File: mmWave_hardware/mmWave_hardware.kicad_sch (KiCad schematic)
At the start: 48 parts, among them J1 Conn_02x08_Top_Bottom, U1 IWRL6432BDBAAMFR, U2 W25Q128JVS, U3 AMS1117-3.3, U4 TPS628502QDRLRQ1, Y1 40.000

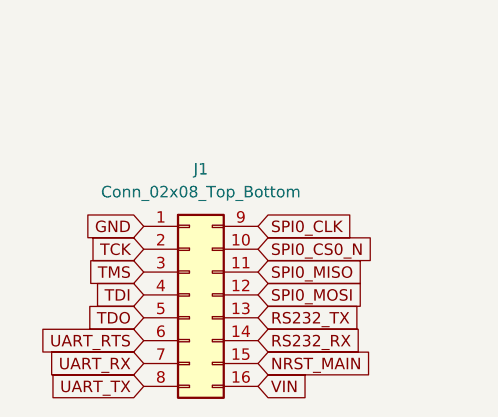
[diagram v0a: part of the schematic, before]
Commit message: PCB Complete
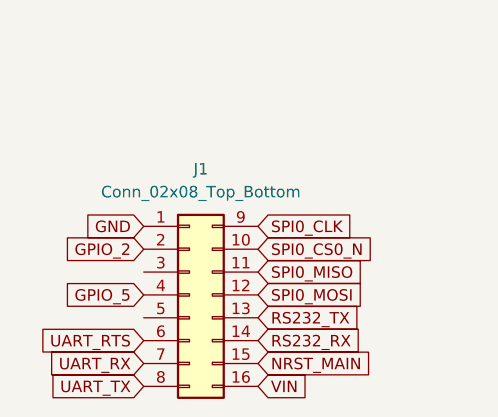
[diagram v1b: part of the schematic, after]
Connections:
- net GPIO_2: now also J1.2 (Pin_2)
- net GPIO_5: now also J1.4 (Pin_4)
- net TCK: no longer J1.2 (Pin_2)
- net TDI: no longer J1.4 (Pin_4)
- net TDO: no longer J1.5 (Pin_5)
- net TMS: no longer J1.3 (Pin_3)

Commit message: pcb
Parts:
- Y1: footprint Crystal:Crystal_SMD_3225-4Pin_3.2x2.5mm_HandSoldering -> Crystal:Crystal_SMD_3225-4Pin_3.2x2.5mm
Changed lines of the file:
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@@
 			)
 		)
-		(property "Footprint" "Crystal:Crystal_SMD_3225-4Pin_3.2x2.5mm_HandSoldering"
+		(property "Footprint" "Crystal:Crystal_SMD_3225-4Pin_3.2x2.5mm"
 			(at 87.63 67.31 0)
 			(effects

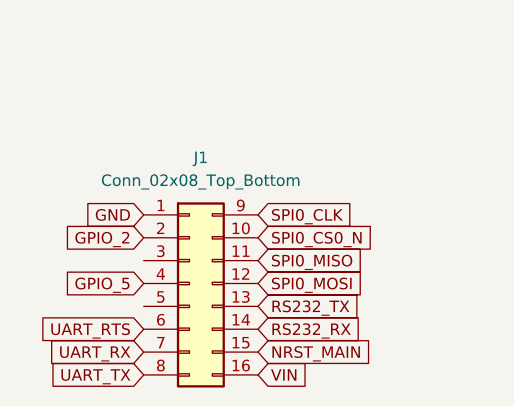
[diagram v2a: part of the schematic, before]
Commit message: PCB Done
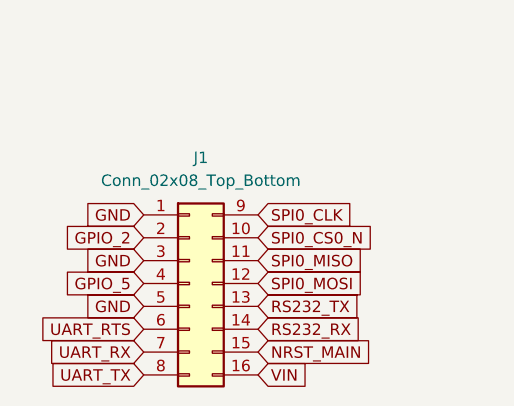
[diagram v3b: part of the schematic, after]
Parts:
- TP1, TP2, TP3, TP4, TP5: footprint TestPoint:TestPoint_Pad_D1.5mm -> TestPoint:TestPoint_Pad_D1.0mm
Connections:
- net GND: now also J1.3 (Pin_3), J1.5 (Pin_5)
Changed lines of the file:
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@@
 		)
 	)
+	(global_label "GND"
+		(shape input)
+		(at 72.39 218.44 180)
+		(fields_autoplaced yes)
+		(effects
+			(font
+				(size 1.27 1.27)
+			)
+			(justify right)
+		)
+		(property "Intersheetrefs" "${INTERSHEET_REFS}"
+			(at 65.5343 218.44 0)
+			(effects
+				(font
+					(size 1.27 1.27)
+				)
+				(justify right)
+				(hide yes)
+			)
+		)
+	)
 	(global_label "VDD_SRAM"
 		(shape input)
@@
 		)
 	)
+	(global_label "GND"
+		(shape input)
+		(at 72.39 213.36 180)
+		(fields_autoplaced yes)
+		(effects
+			(font
+				(size 1.27 1.27)
+			)
+			(justify right)
+		)
+		(property "Intersheetrefs" "${INTERSHEET_REFS}"
+			(at 65.5343 213.36 0)
+			(effects
+				(font
+					(size 1.27 1.27)
+				)
+				(justify right)
+				(hide yes)
+			)
+		)
+	)
 	(global_label "UART_RX"
 		(shape input)
@@
 			)
 		)
-		(property "Footprint" "TestPoint:TestPoint_Pad_D1.5mm"
+		(property "Footprint" "TestPoint:TestPoint_Pad_D1.0mm"
 			(at 300.99 106.68 0)
 			(effects
@@
 			)
 		)
-		(property "Footprint" "TestPoint:TestPoint_Pad_D1.5mm"
+		(property "Footprint" "TestPoint:TestPoint_Pad_D1.0mm"
 			(at 300.99 111.76 0)
 			(effects
@@
 			)
 		)
-		(property "Footprint" "TestPoint:TestPoint_Pad_D1.5mm"
+		(property "Footprint" "TestPoint:TestPoint_Pad_D1.0mm"
 			(at 275.59 97.79 0)
 			(effects
@@
 			)
 		)
-		(property "Footprint" "TestPoint:TestPoint_Pad_D1.5mm"
+		(property "Footprint" "TestPoint:TestPoint_Pad_D1.0mm"
 			(at 127 87.63 0)
 			(effects
@@
 			)
 		)
-		(property "Footprint" "TestPoint:TestPoint_Pad_D1.5mm"
+		(property "Footprint" "TestPoint:TestPoint_Pad_D1.0mm"
 			(at 275.59 102.87 0)
 			(effects

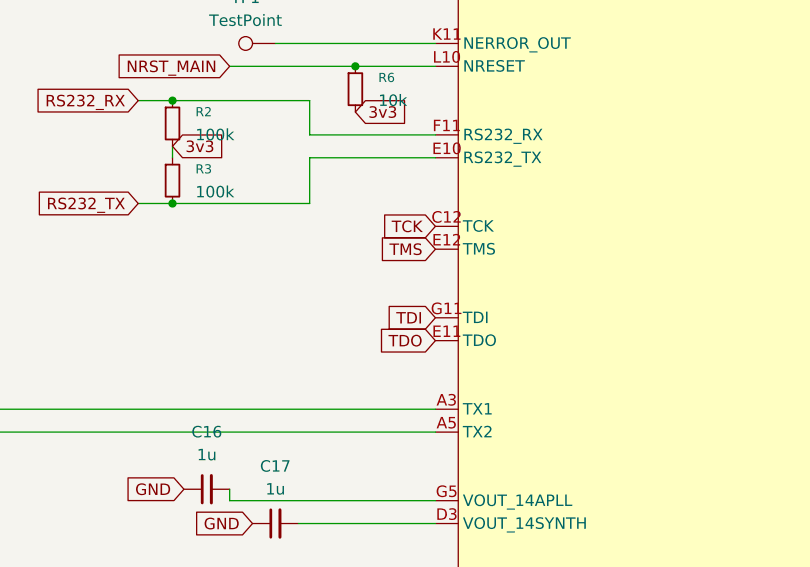
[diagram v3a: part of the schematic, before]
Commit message: PCB
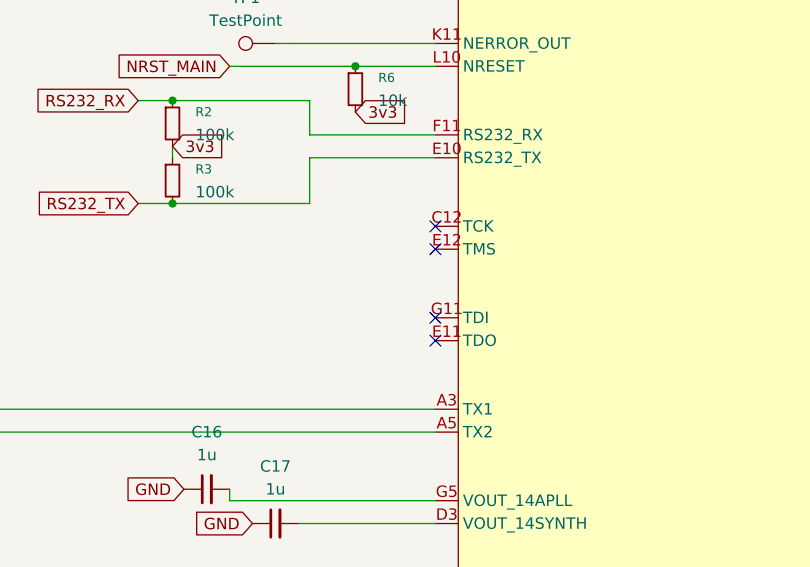
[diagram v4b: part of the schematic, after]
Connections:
- net TCK: no longer names the net of U1.C12 (TCK)
- net TDI: no longer names the net of U1.G11 (TDI)
- net TDO: no longer names the net of U1.E11 (TDO)
- net TMS: no longer names the net of U1.E12 (TMS)
- no-connect marks 2 -> 6

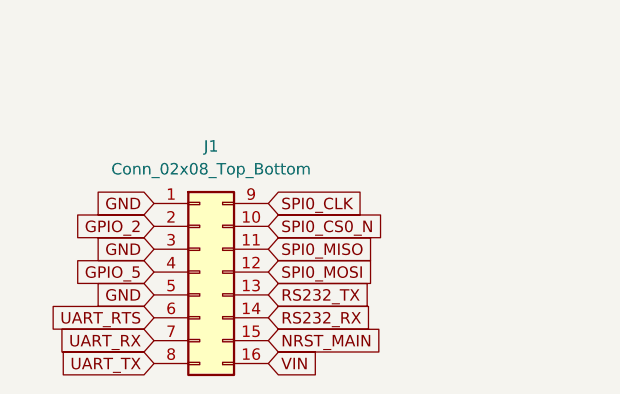
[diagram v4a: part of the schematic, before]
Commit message: routing done
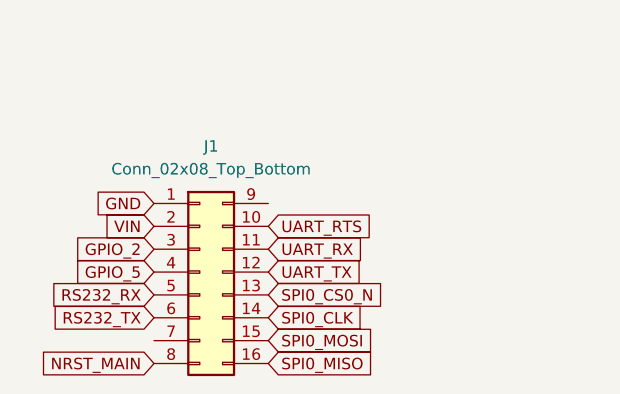
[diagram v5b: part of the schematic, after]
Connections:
- net GND: no longer J1.3 (Pin_3), J1.5 (Pin_5)
- net GPIO_2: now also J1.3 (Pin_3); no longer J1.2 (Pin_2)
- net NRST_MAIN: now also J1.8 (Pin_8); no longer J1.15 (Pin_15)
- net RS232_RX: now also J1.5 (Pin_5); no longer J1.14 (Pin_14)
- net RS232_TX: now also J1.6 (Pin_6); no longer J1.13 (Pin_13)
- net SPI0_CLK: now also J1.14 (Pin_14); no longer J1.9 (Pin_9)
- net SPI0_CS0_N: now also J1.13 (Pin_13); no longer J1.10 (Pin_10)
- net SPI0_MISO: now also J1.16 (Pin_16); no longer J1.11 (Pin_11)
- net SPI0_MOSI: now also J1.15 (Pin_15); no longer J1.12 (Pin_12)
- net UART_RTS: now also J1.10 (Pin_10); no longer J1.6 (Pin_6)
- net UART_RX: now also J1.11 (Pin_11); no longer J1.7 (Pin_7)
- net UART_TX: now also J1.12 (Pin_12); no longer J1.8 (Pin_8)
- net VIN: now also J1.2 (Pin_2); no longer J1.16 (Pin_16)
